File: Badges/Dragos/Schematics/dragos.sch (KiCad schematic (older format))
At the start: 31 parts, among them J1 Conn_01x02, J2 Left, J3 Right, J4 Conn_01x02, J5 Prog, J7 USB_C_Receptacle, SW1 SW_DIP_x01, SW2 Prog, SW3 Power, U1 STM32F042F6Px, U2 TLV1117-33, U3 HX4056, Y1 8MHz

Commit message: Progress on Dragos badge
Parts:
- removed J1, J4: Conn_01x02, Connector_PinHeader_2.54mm:PinHeader_1x02_P2.54mm_Vertical, symbol badge-rescue:Conn_01x02
- removed J2: Left, Connector_PinHeader_2.54mm:PinHeader_1x05_P2.54mm_Vertical, symbol Connector_Generic:Conn_01x05
- removed J3: Right, Connector_PinHeader_2.54mm:PinHeader_1x06_P2.54mm_Vertical, symbol Connector_Generic:Conn_01x06
- removed J5: Prog, Connector_PinHeader_2.54mm:PinHeader_1x04_P2.54mm_Vertical, symbol badge-rescue:Conn_01x04
- removed R4: 0ohm, Resistors_SMD:R_0805_HandSoldering, symbol badge-rescue:R
- removed SW2: Prog, BreadBoardPwr:SK-3296S_switch, symbol Switch:SW_SPDT
- removed U1: STM32F042F6Px, Package_SO:TSSOP-20_4.4x6.5mm_P0.65mm, symbol MCU_ST_STM32F0:STM32F042F6Px
- removed Y1: 8MHz, Crystal:Crystal_SMD_5032-2Pin_5.0x3.2mm, symbol Device:Crystal_Small
- added C12: 100nF, Capacitor_SMD:C_0805_2012Metric, symbol Device:C_Small
- added C13: 1uF, Capacitor_SMD:C_0805_2012Metric, symbol Device:C_Small
- added C14: 4.7uF, Capacitor_SMD:C_0805_2012Metric, symbol Device:C_Small
- added C15, C16: 10pF, Capacitor_SMD:C_0805_2012Metric, symbol Device:C_Small
- added C17, C18: 2.2pF, Capacitor_SMD:C_0805_2012Metric, symbol Device:C_Small
- added D1, D2: LED, LED_SMD:LED_0603_1608Metric, symbol Device:LED
- added D3: LED_ALT, symbol Device:LED_ALT
- added J1: One, Connector_PinHeader_2.54mm:PinHeader_1x08_P2.54mm_Vertical, symbol Connector_Generic:Conn_01x08
- added J2: Two, Connector_PinHeader_2.54mm:PinHeader_1x11_P2.54mm_Vertical, symbol Connector_Generic:Conn_01x11
- added J3: CC2530-ISP, Connector_PinHeader_2.54mm:PinHeader_2x05_P2.54mm_Vertical, symbol Connector_Generic:Conn_02x05_Odd_Even
- added J4: Three, Connector_PinHeader_2.54mm:PinHeader_1x14_P2.54mm_Vertical, symbol Connector_Generic:Conn_01x14
- added J5: Prog, Connector_PinHeader_2.54mm:PinHeader_1x06_P2.54mm_Vertical, symbol Connector_Generic:Conn_01x06
- added J6: Oled_FFS, Connector_FFC-FPC:TE_1-84953-0_1x10-1MP_P1.0mm_Horizontal, symbol Connector_Generic:Conn_01x11
- added J8: Four, Connector_PinHeader_2.54mm:PinHeader_1x13_P2.54mm_Vertical, symbol Connector_Generic:Conn_01x13
- added J9: BreadboardPwr, Connector_PinHeader_2.54mm:PinHeader_1x02_P2.54mm_Vertical, symbol Connector_Generic:Conn_01x02
- added L1: L_Small, Inductor_SMD:L_0603_1608Metric, symbol Device:L_Small
- added R10, R13, R14, R4, R7, R8: 4k7, Resistor_SMD:R_0805_2012Metric, symbol Device:R_Small
- added R11, R12: 330Ohm, Resistor_SMD:R_0805_2012Metric, symbol Device:R_Small
- added R9: 1k, Resistor_SMD:R_0805_2012Metric, symbol Device:R_Small
- added SW2, SW4: SW_DIP_x01, Dragos:1TS002E-2500-2500-CT-HYP-Button, symbol Switch:SW_DIP_x01
- added U1: STM32F411RETx, Package_QFP:LQFP-64_10x10mm_P0.5mm, symbol MCU_ST_STM32F4:STM32F411RETx
- added U4: EByte-CC2530, RF_Module:E18-MS1-PCB, symbol Dragos:EByte-CC2530
- added U5: K1-5202UA-03(5Way_Switch), Dragos:K1-5202UA-03(5way-switch), symbol Dragos:K1-5202UA-03(5Way_Switch)
- added Y1: 12MHz, Crystal:Crystal_SMD_SeikoEpson_TSX3225-4Pin_3.2x2.5mm, symbol Device:Crystal_GND24
- added Y2: 32.768kHz, Crystal:Crystal_SMD_3215-2Pin_3.2x1.5mm, symbol Device:Crystal_Small
- C1, C2: value 20pF -> 100nF
- C4: value 4.7uF -> 100nF
- C6: value 1uF -> 4.7uF
- C7: value 10nF -> 100nF
- R3: value 10k -> 100k
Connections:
- net labels added: Boot0, PA11, PA12, PA13, PA14, PA15, PA8, PB0, PB10, PB12, PB13, PB14, PB15, PB2, PB3, PB4, PB5, PB6, PB7, PB8, PB9, PC0, PC1, PC10, PC11, PC12, PC13, PC2, PC3, PC4, PC5, PC6, PC7, PC8, PC9, PD2
- net labels removed: BOOT0, PF0, PF1, Stat1, Stat2
- wire segments 73 -> 152
- no-connect marks 11 -> 32
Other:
- note added: "Battery Charger IC\n"
- note added: "Boot1"
- note added: "Eye Light, Reverse mount LED"
- note added: "Filter Caps\n"
- note added: "I2C Pullups"
- note added: "Voltage Regulation"
- moved on the sheet: BT1, C10, C11, C8, C9, J7, R1, R2, R5, R6, SW3, U2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

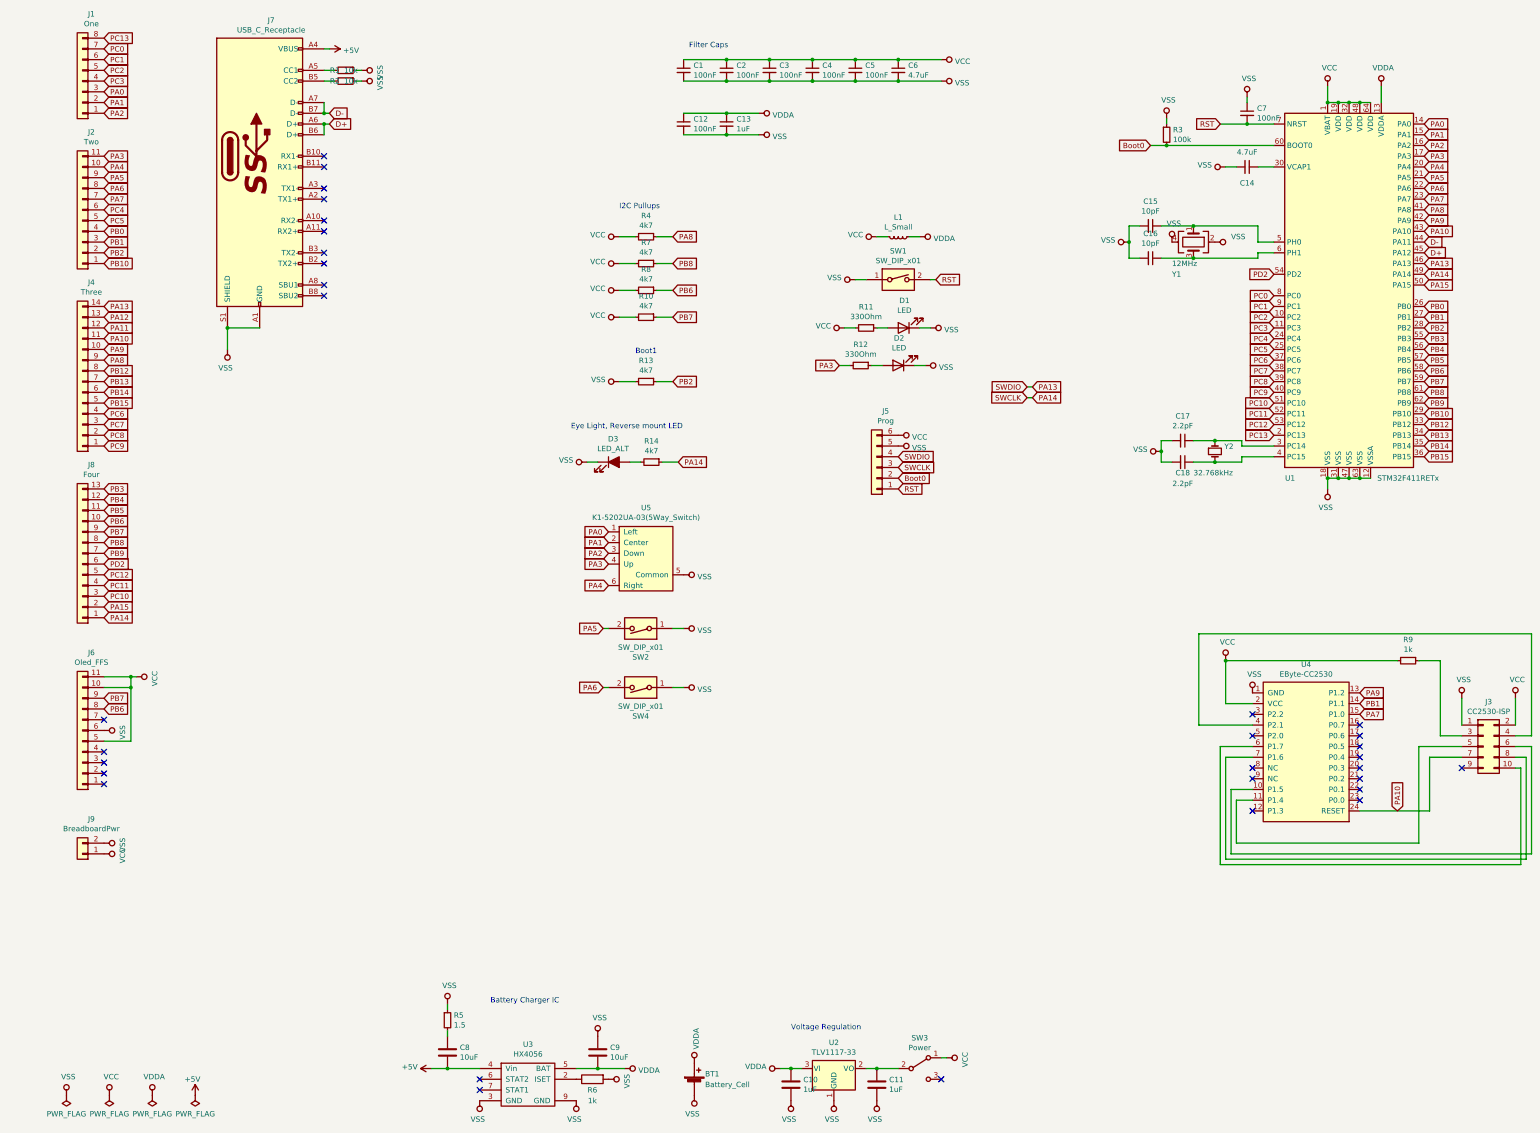
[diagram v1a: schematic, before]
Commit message: Almost done
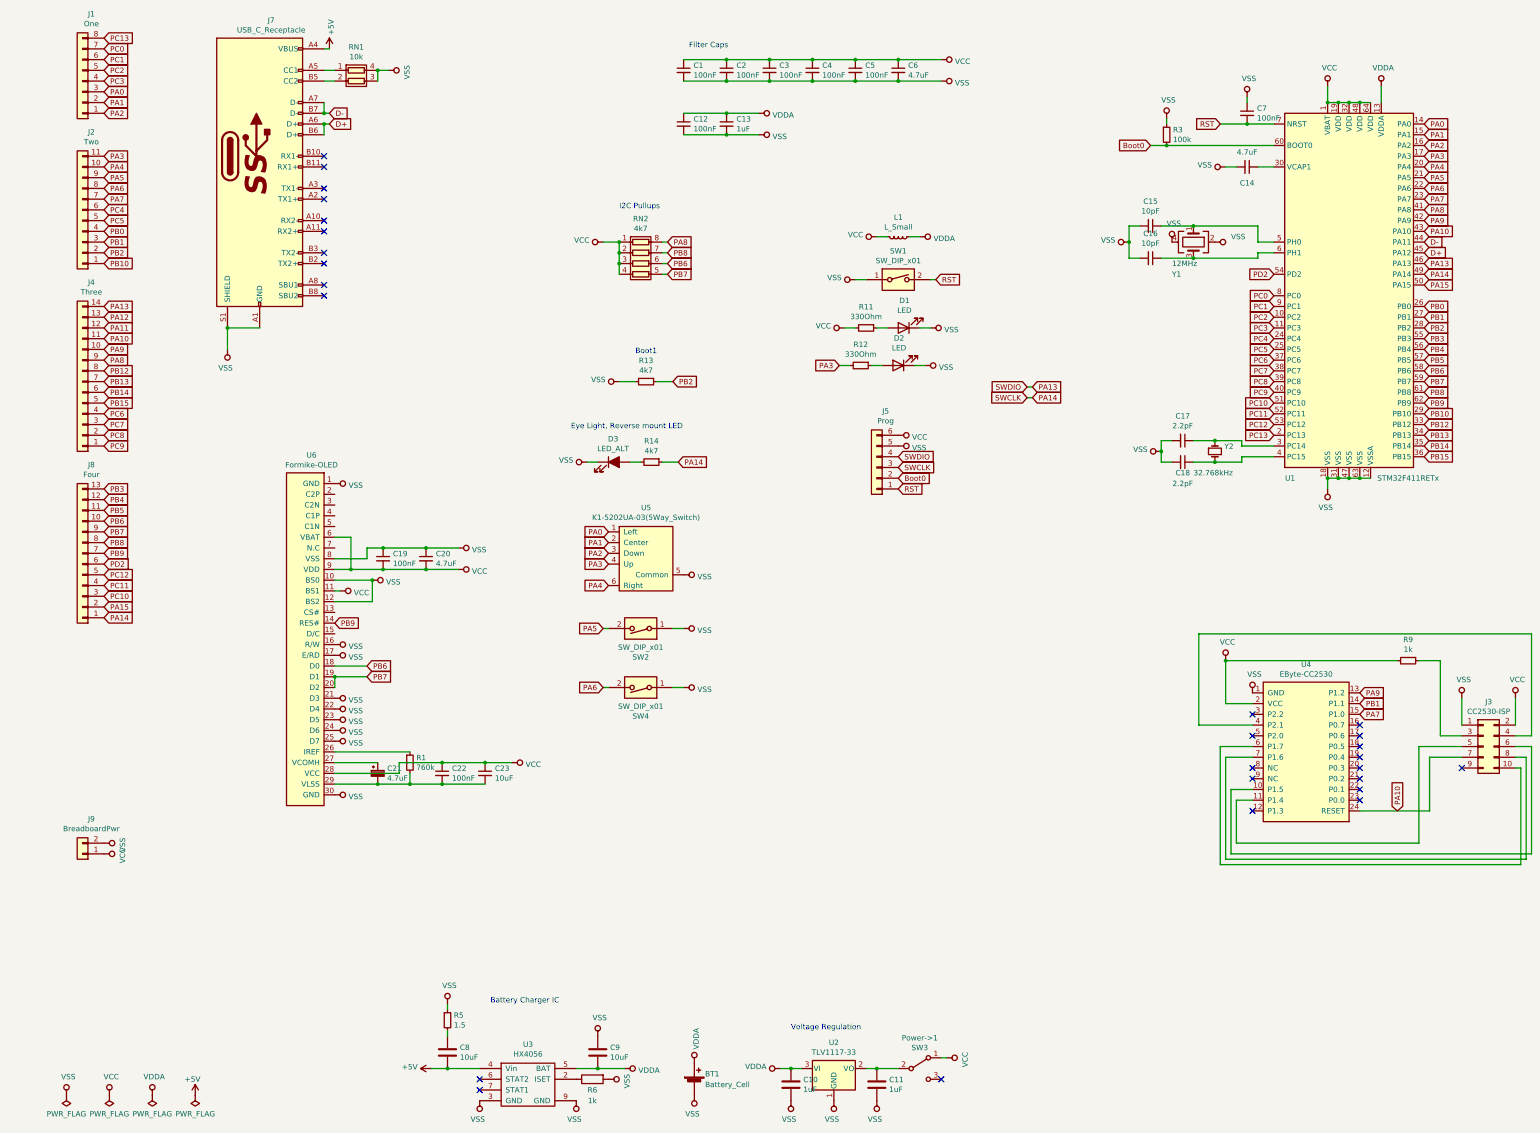
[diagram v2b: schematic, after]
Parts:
- removed J6: Oled_FFS, Connector_FFC-FPC:TE_1-84953-0_1x10-1MP_P1.0mm_Horizontal, symbol Connector_Generic:Conn_01x11
- removed R10, R4, R7, R8: 4k7, Resistor_SMD:R_0805_2012Metric, symbol Device:R_Small
- removed R2: 10k, Resistor_SMD:R_0805_2012Metric, symbol Device:R_Small
- added C19, C22: 100nF, Capacitor_SMD:C_0805_2012Metric, symbol Device:C_Small
- added C20: 4.7uF, Capacitor_SMD:C_0805_2012Metric, symbol Device:C_Small
- added C21: 4.7uF, Capacitor_SMD:C_2010_5025Metric_Pad1.52x2.65mm_HandSolder, symbol Device:CP_Small
- added C23: 10uF, Capacitor_SMD:C_0805_2012Metric, symbol Device:C_Small
- added RN1: 10k, Resistor_SMD:R_Array_Concave_2x0603, symbol Device:R_Pack02
- added RN2: 4k7, Resistor_SMD:R_Array_Concave_4x0603, symbol Device:R_Pack04
- added U6: Formike-OLED, symbol Dragos:Formike-OLED
- D3: footprint (none) -> Dragos:T776-ReverseMountLED
- Power->1: renamed from SW3; value Power -> SW3
- R1: value 10k -> 760k
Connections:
- net PA8: now also RN2.8 (R1.2)
- net PB6: now also RN2.6 (R3.2), U6.18 (D0)
- net PB7: now also RN2.5 (R4.2), U6.19 (D1), U6.20 (D2)
- net PB8: now also RN2.7 (R2.2)
- net PB9: now also U6.14 (RES#)
- net VCC: now also C19.2, C20.2, C22.1, C23.1, RN2.1 (R1.1), RN2.2 (R2.1), RN2.3 (R3.1), RN2.4 (R4.1), U6.11 (BS1), U6.28 (VCC), U6.6 (VBAT), U6.9 (VDD)
- net VSS: now also C19.1, C20.1, RN1.3 (R2.2), RN1.4 (R1.2), U6.1 (GND), U6.10 (BS0), U6.12 (BS2), U6.16 (R/W), U6.17 (E/RD), U6.21 (D3), U6.22 (D4), U6.23 (D5), U6.24 (D6), U6.25 (D7), U6.30 (GND), U6.8 (VSS); no longer R1.1
- net at J7.A5 (CC1): now also RN1.1 (R1.1); no longer R1.2
- net at J7.B5 (CC2): now also RN1.2 (R2.1)
- new net: R1.1, U6.26 (IREF)
- new net: C21.1, U6.27 (VCOMH)
- new net: C21.2, C22.2, C23.2, R1.2, U6.29 (VLSS)
- no-connect marks 32 -> 27
